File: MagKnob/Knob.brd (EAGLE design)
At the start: 36.3 x 29.8 mm, 10 parts, among them SW1 TopUp EC12PLRGBSDVBF-D, U1 attiny841-ssur, U2 EXCLUDE

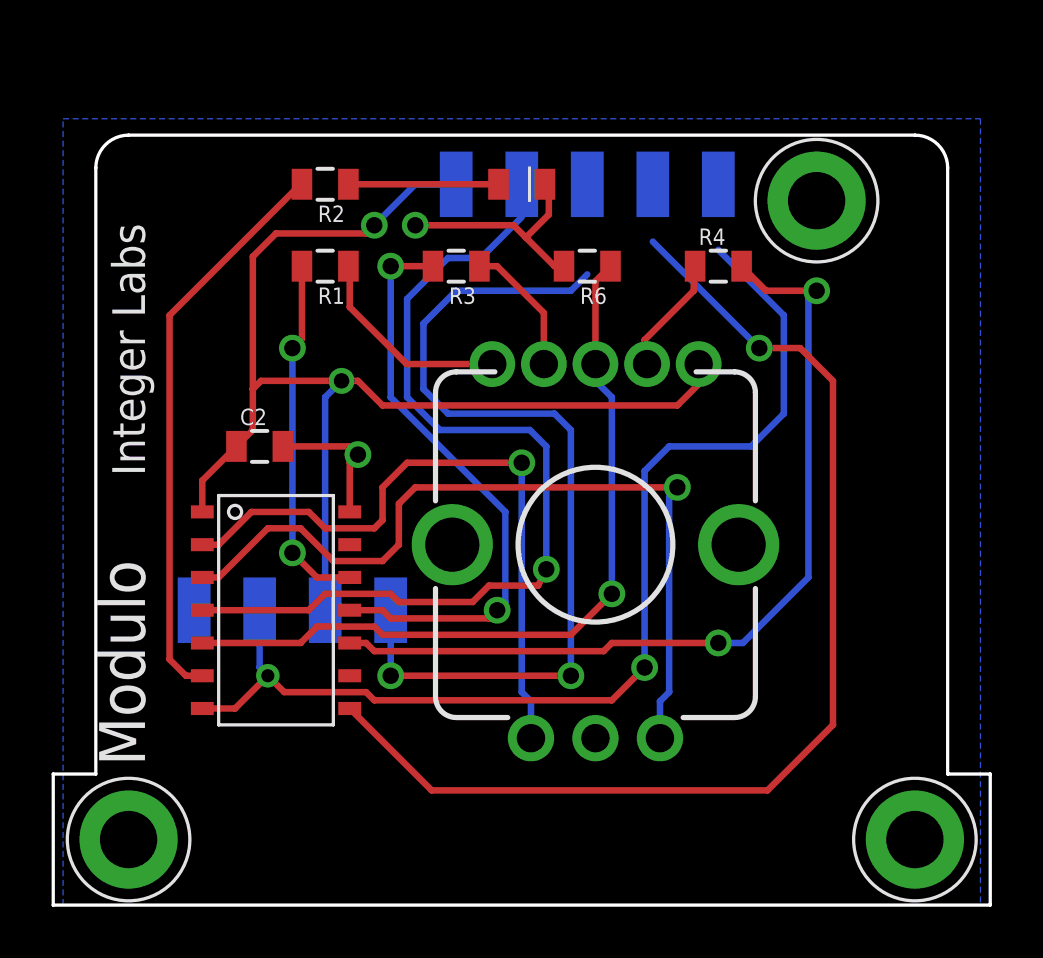
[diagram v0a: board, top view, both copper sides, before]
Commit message: Checkpointing PCB designs
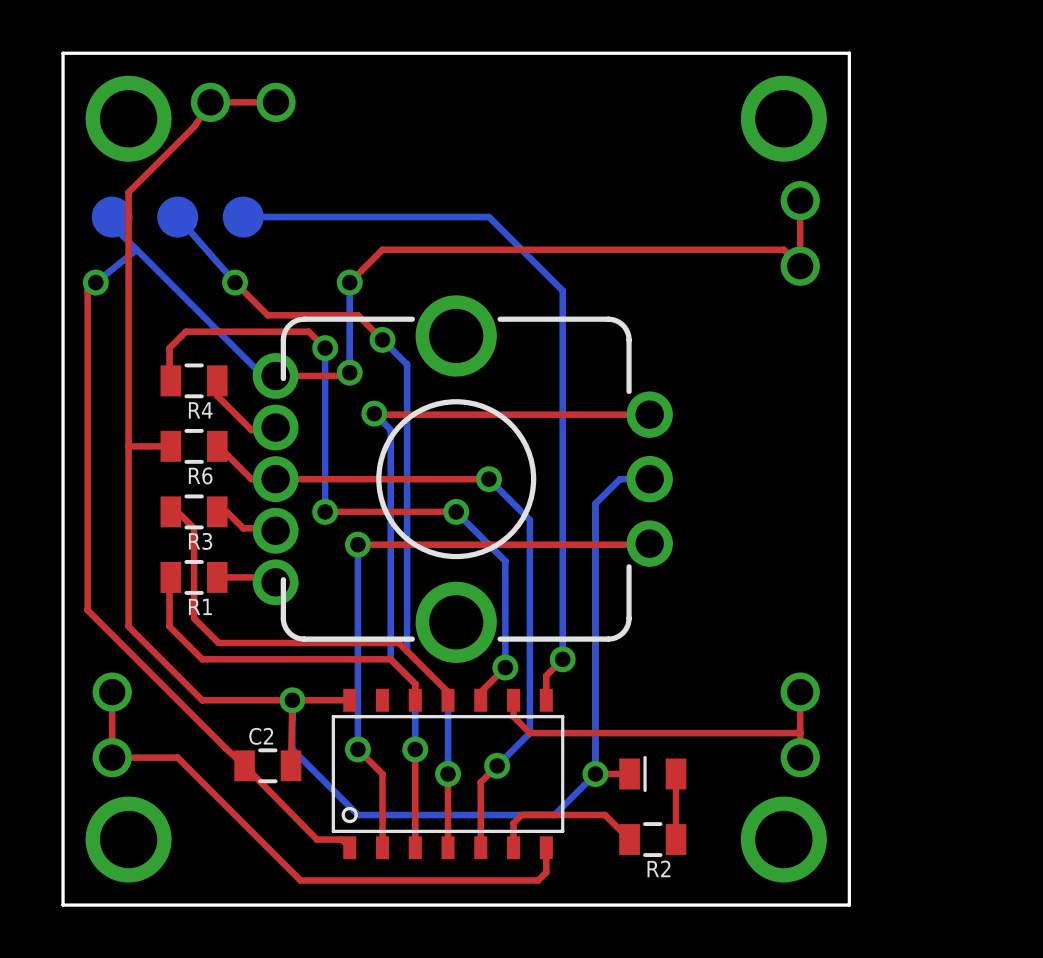
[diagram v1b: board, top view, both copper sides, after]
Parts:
- removed U2: EXCLUDE, Modulo:DEVICE-PCB
- added PCB1: MAGDEVICE, Modulo:MAGDEVICE
- moved R2 28.4 mm to (22.9, 2.54)
- moved LED1 23.4 mm to (22.9, 5.08), turned to 90 degrees
- moved R4 20.8 mm to (5.08, 20.3), turned to 180 degrees
- moved R6 16.8 mm to (5.08, 17.8)
- moved R3 13.9 mm to (5.08, 15.2)
- moved R1 13.1 mm to (5.08, 12.7)
- moved C2 12.4 mm to (7.94, 5.40)
- moved U1 10.2 mm to (11.1, 5.40), turned to 0 degrees
- moved SW1 5.97 mm to (15.2, 16.5), turned to 90 degrees
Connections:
- net GND: now also PCB1.GNDA, PCB1.GNDB; no longer U2.BUS0
- net MISO: now also PCB1.MISO; no longer U2.PROG3
- net RESET: now also PCB1.RESET; no longer U2.PROG1
- net SCL/SCK: now also PCB1.SCLA, PCB1.SCLB; no longer U2.BUS3, U2.PROG2
- net SDA/MOSI: now also PCB1.SDAA, PCB1.SDAB; no longer U2.BUS1, U2.PROG4
- net VCC: now also PCB1.VCCA, PCB1.VCCB, PCB1.VPROG; no longer U2.BUS2, U2.PROG0
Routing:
- net GND: track 14.4 -> 67.7 mm
- net SCL/SCK: track 35.1 -> 14.6 mm, vias 2 -> 0
- net SDA/MOSI: track 42.6 -> 22.4 mm, vias 2 -> 0
- net VCC: track 47.8 -> 65.6 mm, vias 2 -> 3
- net LED: track 22.2 -> 5.98 mm
- net MISO: track 43.7 -> 29.7 mm
- net GREEN: track 22.9 -> 16.0 mm, vias 2 -> 0
- net BLUE: track 33.6 -> 27.8 mm, vias 2 -> 4
- net N$4: track 8.05 -> 2.34 mm
- net RESET: track 34.9 -> 30.7 mm, vias 1 -> 3
- net B: track 31.8 -> 28.2 mm, vias 1 -> 2
- net SW: track 30.1 -> 26.8 mm, vias 1 -> 2
- net N$7: track 5.82 -> 2.54 mm
- net N$5: track 5.23 -> 2.54 mm
- net A: track 25.8 -> 23.5 mm, vias 1 -> 2
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- removed copper zone on layer 16, net GND
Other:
- board size 36.3 x 29.8 mm -> 30.5 x 33 mm
